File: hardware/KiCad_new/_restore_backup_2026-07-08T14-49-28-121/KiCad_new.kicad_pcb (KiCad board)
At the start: 2 copper layers, 50 x 76.2 mm, 26 parts, among them J1 J1 Power, J2 J2 NTC, J3 Meter, J4 Relay Module, J5 Control Panel, U1 ESP32-C3 Dev Board, U2 AMS1117

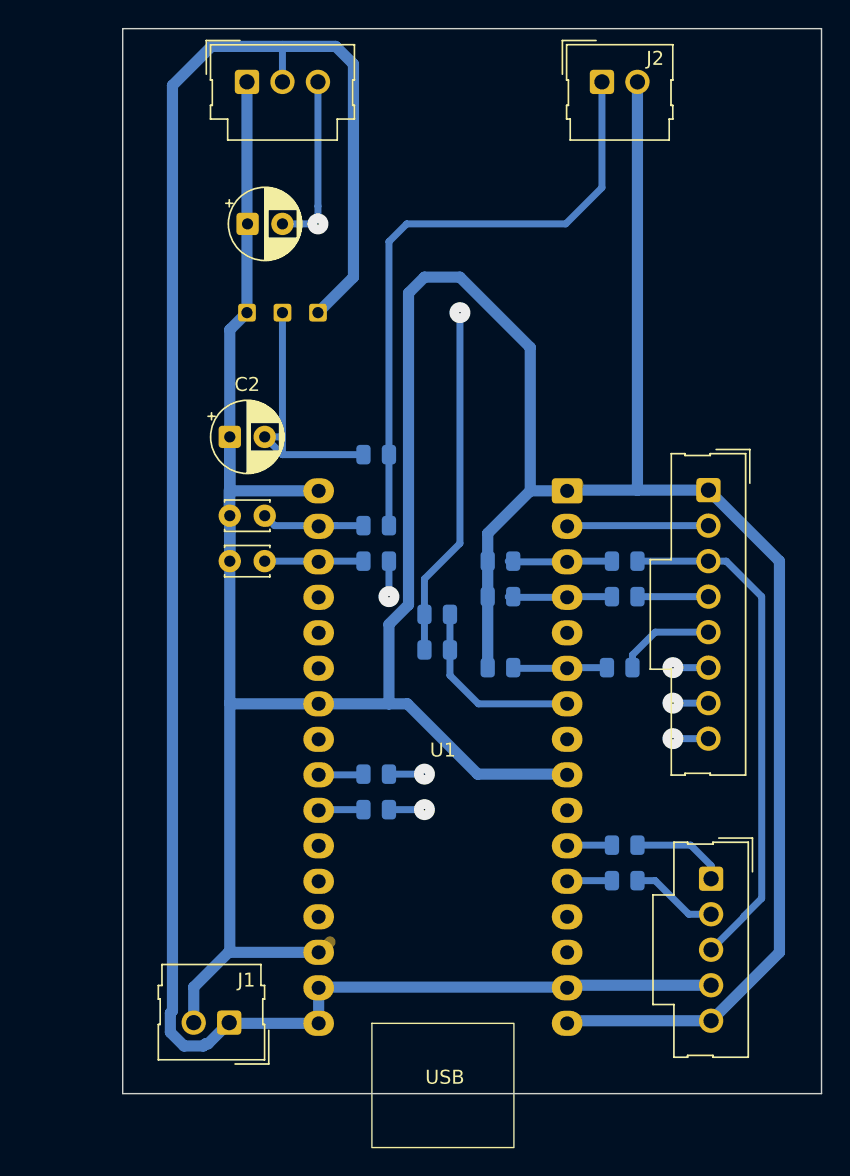
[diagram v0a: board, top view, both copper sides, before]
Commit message: Create PCB
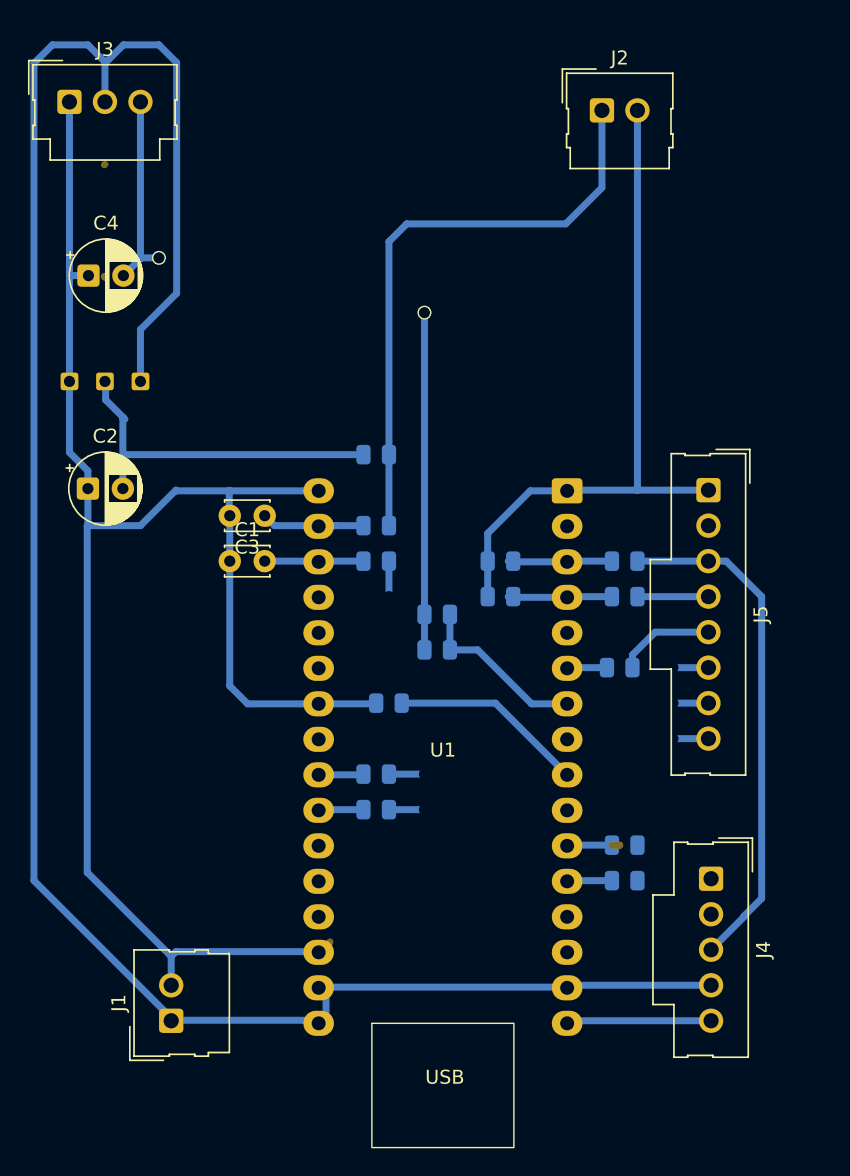
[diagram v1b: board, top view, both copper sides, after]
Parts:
- moved U2 13.6 mm to (88.9, 81.1)
- moved J3 12.8 mm to (86.4, 62.4)
- moved C4 12.0 mm to (87.7, 74.8)
- moved C2 10.8 mm to (87.7, 90.1)
- moved R5 8.37 mm to (109.2, 105.4), turned to 0 degrees
- moved J1 4.15 mm to (93.6, 128.1), turned to 90 degrees
- moved J2 2.04 mm to (124.5, 63.0)
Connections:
- R6 pad 2: Net-(J4-Pin_1) -> Net-(J4-Pin_2)
- R7 pad 2: Net-(J4-Pin_2) -> Net-(J4-Pin_1)
- U1 pad 2: Net-(J5-Pin_2) -> unconnected-(U1-+3.3v-Pad2)
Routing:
- net GND: track 277.8 -> 195.3 mm
- net Net-(J5-Pin_2): track 10.1 -> 0.00 mm
- net Net-(J1-Pin_1): track 146.9 -> 153.7 mm
- net Net-(J4-Pin_1): track 6.82 -> 0.00 mm
- net Net-(U2-VOut_3.3v): track 19.0 -> 25.5 mm
- net Net-(J4-Pin_2): track 6.27 -> 0.00 mm
- net Net-(U1-GPIO6): track 6.75 -> 2.87 mm
- net Net-(J2-Pin_1): track 44.7 -> 42.7 mm
- net Net-(U1-GPIO7): track 13.6 -> 12.5 mm
- net Net-(J3-Pin_3): track 37.9 -> 38.5 mm
- net Net-(U1-GPIO5): track 3.23 -> 3.85 mm
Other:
- board outline removed
